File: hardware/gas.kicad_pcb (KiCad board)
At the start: 2 copper layers, 50 x 30 mm, 41 parts, among them P1 CON-SENSOR2, P10 3, P2 DEBUG, P3 BOOT, P7 0, P8 1, P9 2, U1 XMC1300, U10 MCP3423, U11 spec-sensor, U2 DRILL, U3 DRILL, U4 DRILL, U5 DRILL, U6 HDC1080, U7 ISL60002, U8 LMP91000, U9 MCP6041

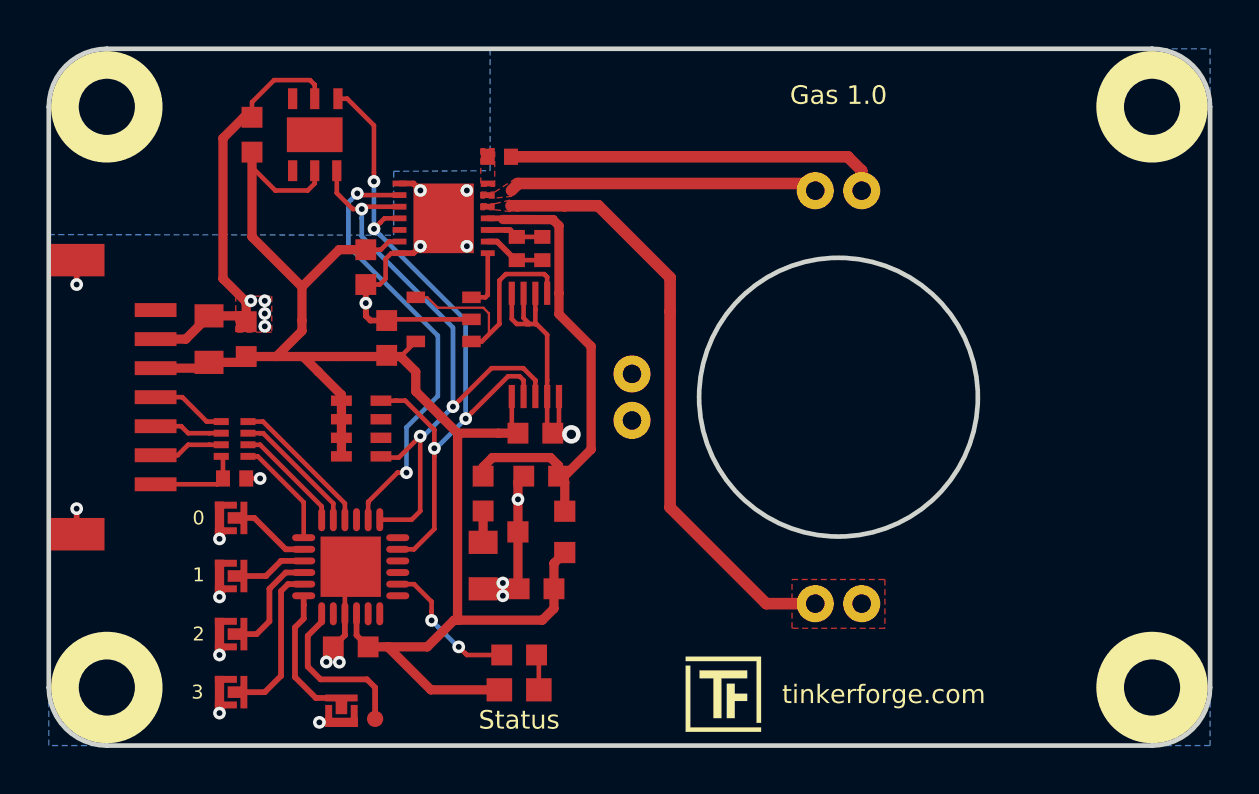
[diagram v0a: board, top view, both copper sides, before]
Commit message: drc check
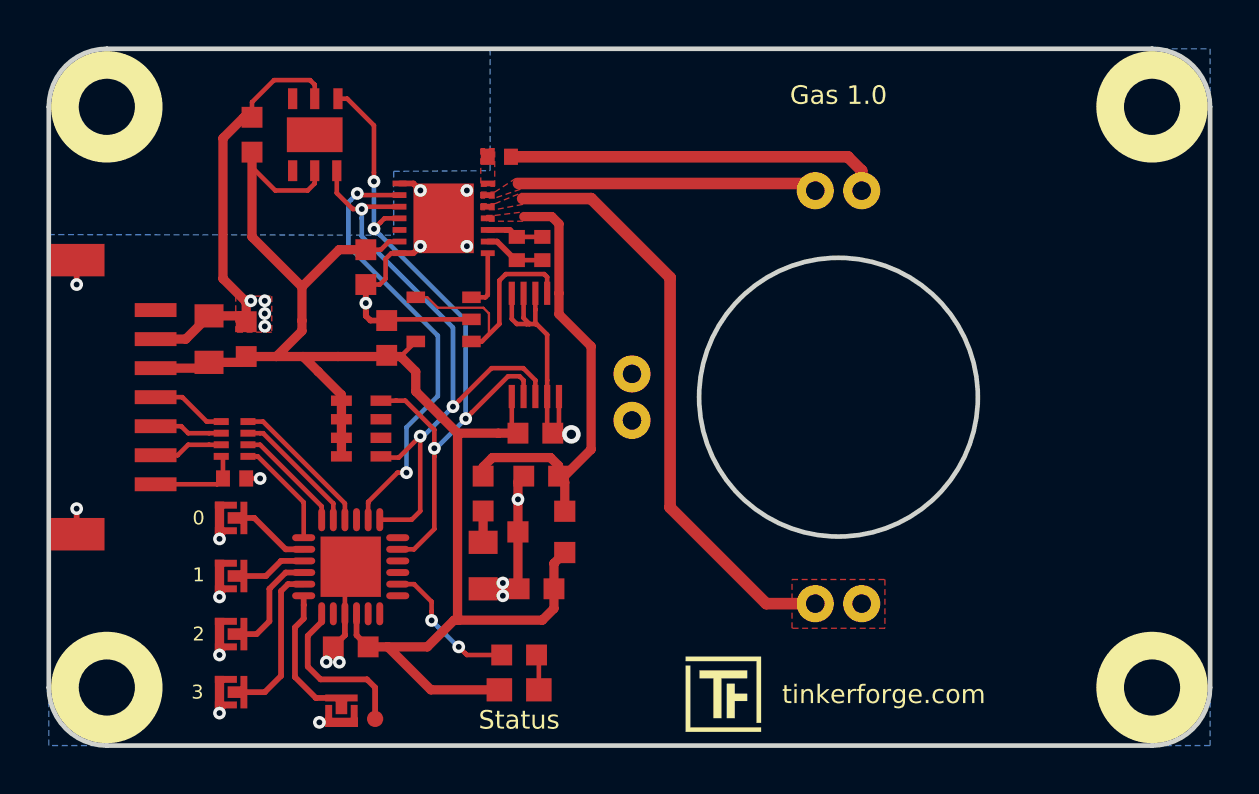
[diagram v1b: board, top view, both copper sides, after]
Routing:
- net Net-(C6-Pad1): track 21.3 -> 19.8 mm
- added copper zone on F.Cu, net Net-(C6-Pad1)
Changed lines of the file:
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@@
     (thickness 1.6)
     (drawings 16)
-    (tracks 403)
+    (tracks 395)
     (zones 0)
     (modules 41)
@@
   (segment (start 143.19888 126.81004) (end 143.79893 126.81004) (width 0.2) (layer F.Cu) (net 36))
   (segment (start 143.79893 126.81004) (end 143.9 126.70897) (width 0.2) (layer F.Cu) (net 36))
-  (segment (start 144.499434 123.41) (end 143.9 123.41) (width 0.25) (layer F.Cu) (net 37))
-  (segment (start 144.55 123.460566) (end 144.499434 123.41) (width 0.25) (layer F.Cu) (net 37))
   (segment (start 147.216 134.776) (end 146.95 134.51) (width 0.4) (layer F.Cu) (net 37))
   (segment (start 147.216 136.021) (end 147.216 134.776) (width 0.4) (layer F.Cu) (net 37))
@@
   (segment (start 146.966 126.6375) (end 146.966 127.53788) (width 0.4) (layer F.Cu) (net 37))
   (segment (start 146.966 127.53788) (end 148.349002 128.920882) (width 0.4) (layer F.Cu) (net 37))
-  (segment (start 146.708019 123.468019) (end 146.700566 123.468019) (width 0.4) (layer F.Cu) (net 37))
-  (segment (start 146.966 123.726) (end 146.708019 123.468019) (width 0.4) (layer F.Cu) (net 37))
-  (segment (start 146.966 126.6375) (end 146.966 123.726) (width 0.4) (layer F.Cu) (net 37))
-  (segment (start 144.55 123.460566) (end 146.700566 123.468019) (width 0.4) (layer F.Cu) (net 37))
-  (segment (start 146.700566 123.468019) (end 146.700566 123.460566) (width 0.4) (layer F.Cu) (net 37))
+  (segment (start 146.966 123.647798) (end 146.966 126.6375) (width 0.4) (layer F.Cu) (net 37))
+  (segment (start 145.45 123.335) (end 146.653202 123.335) (width 0.4) (layer F.Cu) (net 37))
+  (segment (start 146.653202 123.335) (end 146.966 123.647798) (width 0.4) (layer F.Cu) (net 37))
   (segment (start 143.65004 128.70996) (end 143.19888 128.70996) (width 0.1) (layer F.Cu) (net 38))
   (segment (start 141.30117 126.81004) (end 141.75113 127.26) (width 0.1) (layer F.Cu) (net 38))
@@
   (segment (start 144.9 120.76) (end 159.4 120.76) (width 0.5) (layer F.Cu) (net 43))
   (segment (start 159.4 120.76) (end 160 121.36) (width 0.5) (layer F.Cu) (net 43))
-  (segment (start 145.178829 122.869009) (end 144.9 122.869009) (width 0.5) (layer F.Cu) (net 44))
-  (segment (start 147.209009 122.869009) (end 145.178829 122.869009) (width 0.5) (layer F.Cu) (net 44))
-  (segment (start 151.75 135.86) (end 151.75 127.41) (width 0.5) (layer F.Cu) (net 44))
-  (segment (start 158 140) (end 155.89 140) (width 0.5) (layer F.Cu) (net 44))
-  (segment (start 155.89 140) (end 151.75 135.86) (width 0.5) (layer F.Cu) (net 44))
-  (segment (start 147.209009 122.869009) (end 148.659009 122.869009) (width 0.5) (layer F.Cu) (net 44))
-  (segment (start 151.75 125.96) (end 151.75 127.41) (width 0.5) (layer F.Cu) (net 44))
-  (segment (start 148.659009 122.869009) (end 151.75 125.96) (width 0.5) (layer F.Cu) (net 44))
-  (segment (start 145.22 121.91) (end 144.91901 122.21099) (width 0.5) (layer F.Cu) (net 45))
+  (segment (start 155.89 140) (end 158 140) (width 0.5) (layer F.Cu) (net 44))
+  (segment (start 151.75 135.86) (end 155.89 140) (width 0.5) (layer F.Cu) (net 44))
+  (segment (start 151.75 125.96) (end 151.75 135.86) (width 0.5) (layer F.Cu) (net 44))
+  (segment (start 145.4 122.56) (end 148.35 122.56) (width 0.5) (layer F.Cu) (net 44))
+  (segment (start 148.35 122.56) (end 151.75 125.96) (width 0.5) (layer F.Cu) (net 44))
+  (segment (start 157.69 121.91) (end 145.22 121.91) (width 0.5) (layer F.Cu) (net 45))
   (segment (start 158 122.22) (end 157.69 121.91) (width 0.5) (layer F.Cu) (net 45))
-  (segment (start 157.69 121.91) (end 145.22 121.91) (width 0.5) (layer F.Cu) (net 45))
   (zone (net 44) (net_name "Net-(U11-Pad1)") (layer F.Cu) (hatch edge 0.508)
     (connect_pads yes (clearance 0.508))
@@
     (connect_pads yes (clearance 0.001))
     (min_thickness 0.1)
-    (fill yes (arc_segments 16) (thermal_gap 0.508) (thermal_bridge_width 0.508))
+    (fill yes (arc_segments 16) (thermal_gap 0.149) (thermal_bridge_width 0.508))
     (polygon
       (pts
-        (xy 143.6 122.28) (xy 144.2 122.28) (xy 145.15 121.66) (xy 144.95 122.46) (xy 144.2 122.54)
+        (xy 143.6 122.28) (xy 144.2 122.28) (xy 145.15 121.66) (xy 145.3 122.16) (xy 144.2 122.54)
         (xy 143.6 122.54)
       )
@@
     (polygon
       (pts
-        (xy 143.6 122.78) (xy 144.21 122.78) (xy 144.88 122.62) (xy 144.88 123.12) (xy 144.2 123.04)
+        (xy 143.6 122.78) (xy 144.21 122.78) (xy 145.35 122.31) (xy 145.4 122.81) (xy 144.2 123.04)
         (xy 143.6 123.04)
       )
     )
+  )
+  (zone (net 37) (net_name "Net-(C6-Pad1)") (layer F.Cu) (hatch edge 0.508)
+    (connect_pads yes (clearance 0.001))
+    (min_thickness 0.1)
+    (fill yes (arc_segments 16) (thermal_gap 0.149) (thermal_bridge_width 0.508))
+    (polygon
+      (pts
+        (xy 143.85 123.285) (xy 144.2 123.285) (xy 145.425 123.135) (xy 145.425 123.535) (xy 144.2 123.535)
+        (xy 143.85 123.535)
+      )
+    )
